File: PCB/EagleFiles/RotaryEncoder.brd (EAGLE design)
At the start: 27.3 x 15.2 mm, 2 parts, among them SW1 ROTARY-ENCODER

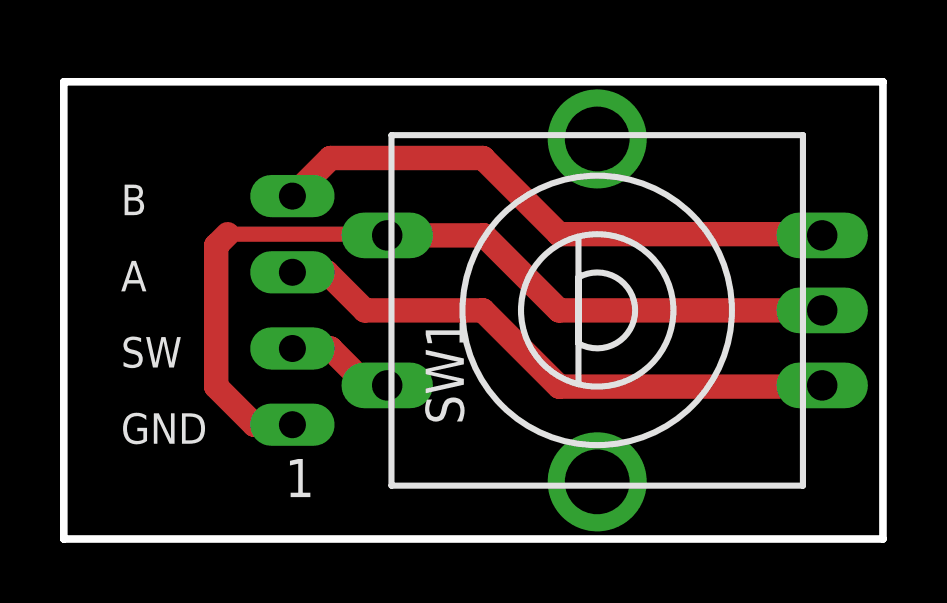
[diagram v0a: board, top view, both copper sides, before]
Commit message: Updated traces
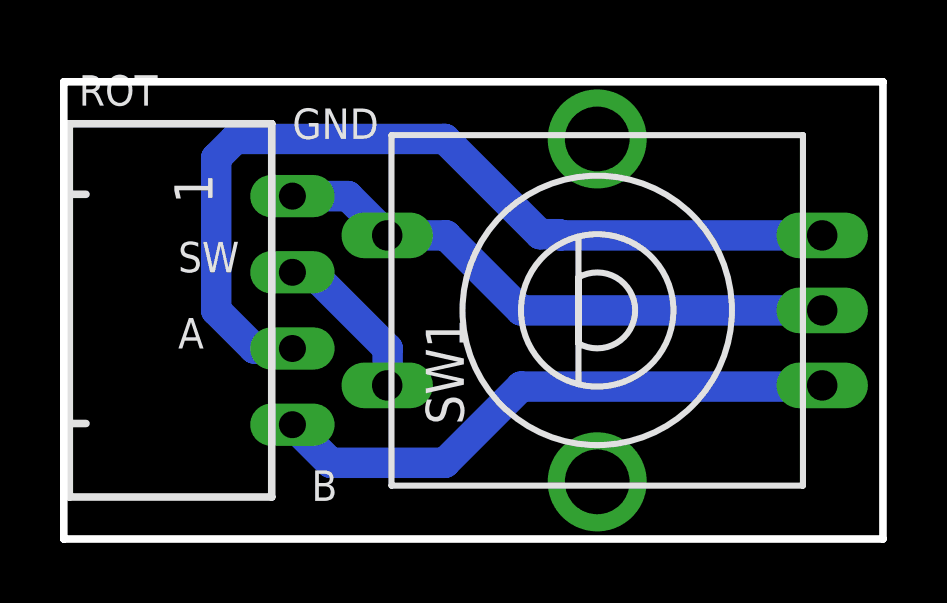
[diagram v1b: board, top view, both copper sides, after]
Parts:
- flipped ROT to the top, turned to 270 degrees
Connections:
- net A: now also SW1.C; no longer SW1.A
- net B: now also SW1.A; no longer SW1.C
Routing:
- net A: track 19.3 -> 29.9 mm
- net GND: track 29.2 -> 19.2 mm
- net SW: track 3.70 -> 5.46 mm
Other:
- board text added: "Components on Top"
- board text removed: "Connector on bottom"
- board text removed: "Rotarty on this side"
